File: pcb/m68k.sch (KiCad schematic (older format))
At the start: 120 parts, among them J1 USB_B_Micro, J2 Mini-DIN-6, J4 DB15_Male_HighDensity, J5 FTSH-105-01-L-DV-K, J6 FTSH-105-01-L-DV-K, J7 FTSH-105-01-L-DV-K, J8 Micro_SD_Card, U1 93LC56, U10 25LCxxx, U11 TXB0108DQSR, U12 TXB0108DQSR, U13 iCE40-HX4K-TQ144, U14 ADV7125KSTZ50, U15 74LVC1G17, U16 LD1117S33TR_SOT223, U17 LD1117S12TR_SOT223, U18 ATL431BQDBZR, U2 68000D, U3 FT2232H, U4 TXB0108DQSR, U5 TXB0108DQSR, U6 TXB0108DQSR, U7 SN74LVC8T245PWR, U8 SN74LVC8T245PWR, U9 AS6C1616, X1 ASV-12.000MHz

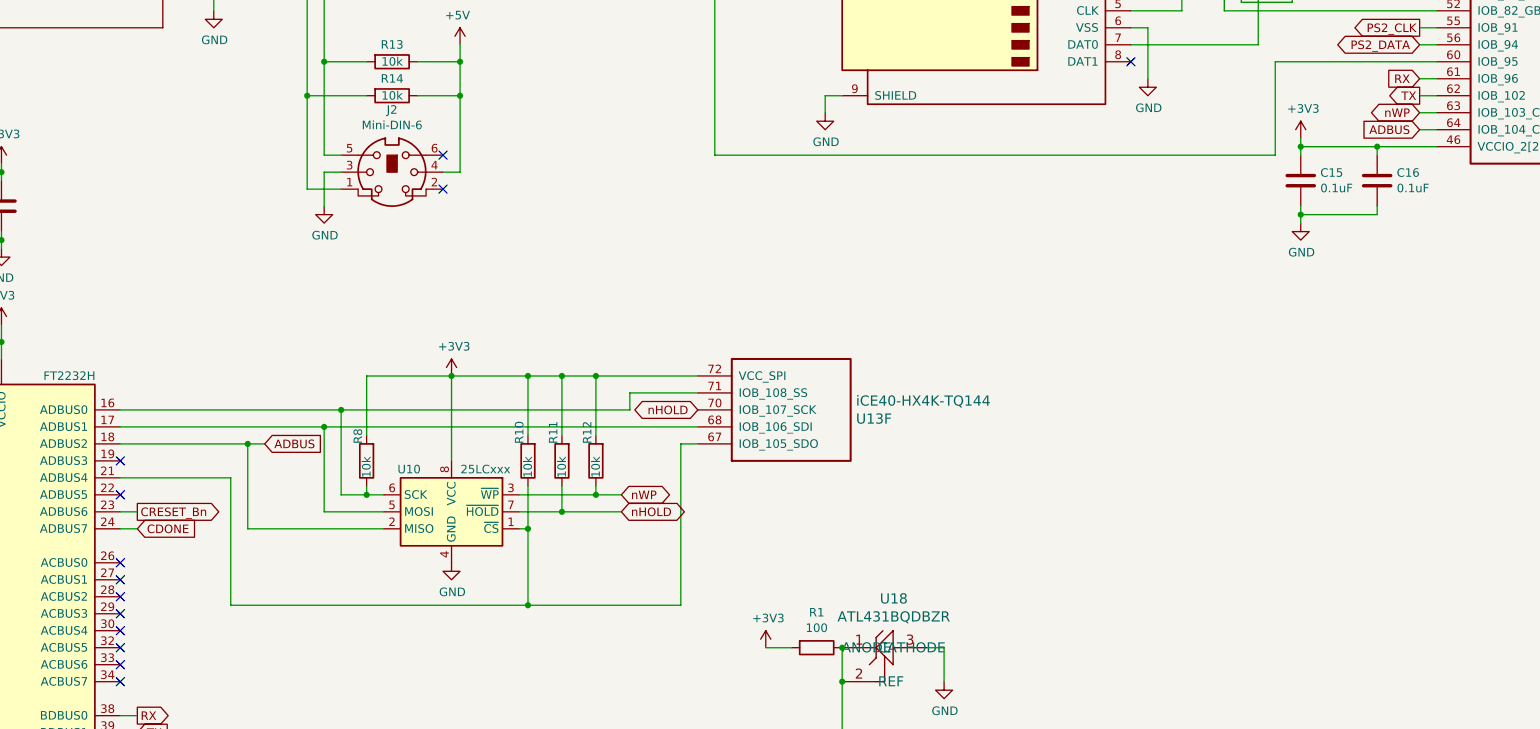
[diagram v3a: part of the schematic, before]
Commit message: almost finish routing
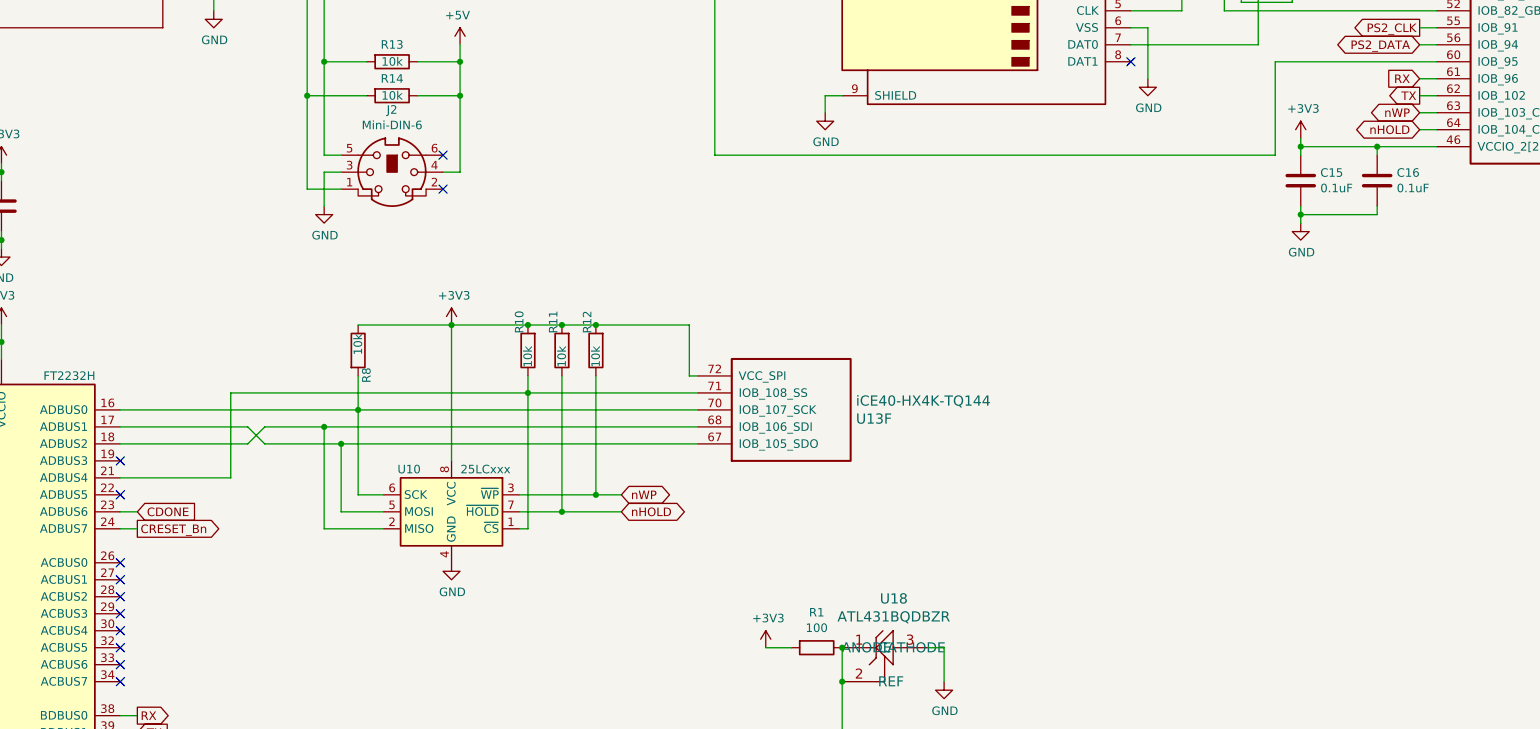
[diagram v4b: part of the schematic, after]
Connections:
- net +3V3: now also R8.1; no longer R8.2
- net CDONE: now also U3.23 (ADBUS6); no longer U3.24 (ADBUS7)
- net CRESET_Bn: now also U3.24 (ADBUS7); no longer U3.23 (ADBUS6)
- net nHOLD: now also U13.64 (IOB_104_CBSEL1); no longer U13.70 (IOB_107_SCK)
- net at R10.1, U10.1 (~CS), U3.21 (ADBUS4): now also U13.71 (IOB_108_SS); no longer U13.67 (IOB_105_SDO)
- net at U10.5 (MOSI), U3.17 (ADBUS1): now also U13.67 (IOB_105_SDO); no longer U13.68 (IOB_106_SDI)
- net at U10.6 (SCK), U3.16 (ADBUS0): now also R8.2, U13.70 (IOB_107_SCK); no longer R8.1, U13.71 (IOB_108_SS)
- net ADBUS: no longer names the net of U10.2 (MISO), U3.18 (ADBUS2)
- net ADBUS: now also U13.68 (IOB_106_SDI); no longer U13.64 (IOB_104_CBSEL1)
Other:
- moved on the sheet: R10, R11, R12, R8
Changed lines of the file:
@@
 Wire Wire Line
 	7200 3500 8050 3500
-Text GLabel 5450 12500 2    50   Input ~ 0
+Text GLabel 5450 12400 2    50   Input ~ 0
 CDONE
 Wire Wire Line
@@
 Wire Wire Line
 	8400 6300 8400 6350
-Text GLabel 13000 10150 0    50   Input ~ 0
-ADBUS
 Wire Wire Line
 	11300 9150 11850 9150
@@
 Wire Wire Line
 	8550 6400 8500 6400
-Wire Wire Line
-	6650 12300 6650 11800
-Text GLabel 6200 12000 2    50   Input ~ 0
-ADBUS
 $Comp
 L Memory_EEPROM:25LCxxx U10
@@
 	1    0    0    -1
 $EndComp
-Text GLabel 5450 12400 2    50   Output ~ 0
+Text GLabel 5450 12500 2    50   Output ~ 0
 CRESET_Bn
 Text GLabel 8300 12300 2    50   BiDi ~ 0
 nWP
-Wire Wire Line
-	7300 12100 7300 11600
-Text GLabel 8750 11800 0    50   BiDi ~ 0
+Text GLabel 13000 10150 0    50   BiDi ~ 0
 nHOLD
 $Comp
 L Device:R R12
 U 1 1 62339B13
-P 8150 12100
-F 0 "R12" V 8200 12000 50  0000 R CNN
-F 1 "10k" V 8150 12200 50  0000 R CNN
-F 2 "Resistor_SMD:R_0603_1608Metric" V 8080 12100 50  0001 C CNN
-F 3 "~" H 8150 12100 50  0001 C CNN
-	1    8150 12100
+P 8150 11450
+F 0 "R12" V 8200 11350 50  0000 R CNN
+F 1 "10k" V 8150 11550 50  0000 R CNN
+F 2 "Resistor_SMD:R_0603_1608Metric" V 8080 11450 50  0001 C CNN
+F 3 "~" H 8150 11450 50  0001 C CNN
+	1    8150 11450
 	-1   0    0    1
 $EndComp
@@
 L Device:R R11
 U 1 1 6233983C
-P 7950 12100
-F 0 "R11" V 8000 12000 50  0000 R CNN
-F 1 "10k" V 7950 12200 50  0000 R CNN
-F 2 "Resistor_SMD:R_0603_1608Metric" V 7880 12100 50  0001 C CNN
-F 3 "~" H 7950 12100 50  0001 C CNN
-	1    7950 12100
+P 7950 11450
+F 0 "R11" V 8000 11350 50  0000 R CNN
+F 1 "10k" V 7950 11550 50  0000 R CNN
+F 2 "Resistor_SMD:R_0603_1608Metric" V 7880 11450 50  0001 C CNN
+F 3 "~" H 7950 11450 50  0001 C CNN
+	1    7950 11450
 	-1   0    0    1
 $EndComp
@@
 L power:+3V3 #PWR0125
 U 1 1 605A3C62
-P 7300 11600
-F 0 "#PWR0125" H 7300 11450 50  0001 C CNN
-F 1 "+3V3" H 7315 11773 50  0000 C CNN
-F 2 "" H 7300 11600 50  0001 C CNN
-F 3 "" H 7300 11600 50  0001 C CNN
-	1    7300 11600
+P 7300 11300
+F 0 "#PWR0125" H 7300 11150 50  0001 C CNN
+F 1 "+3V3" H 7315 11473 50  0000 C CNN
+F 2 "" H 7300 11300 50  0001 C CNN
+F 3 "" H 7300 11300 50  0001 C CNN
+	1    7300 11300
 	1    0    0    -1
 $EndComp
@@
 L Device:R R8
 U 1 1 605A381A
-P 6800 12100
-F 0 "R8" V 6850 12000 50  0000 R CNN
-F 1 "10k" V 6800 12200 50  0000 R CNN
-F 2 "Resistor_SMD:R_0603_1608Metric" V 6730 12100 50  0001 C CNN
-F 3 "~" H 6800 12100 50  0001 C CNN
-	1    6800 12100
-	-1   0    0    1
+P 6750 11450
+F 0 "R8" V 6800 11350 50  0000 R CNN
+F 1 "10k" V 6750 11550 50  0000 R CNN
+F 2 "Resistor_SMD:R_0603_1608Metric" V 6680 11450 50  0001 C CNN
+F 3 "~" H 6750 11450 50  0001 C CNN
+	1    6750 11450
+	1    0    0    -1
 $EndComp
 $Comp
 L Device:R R10
 U 1 1 605A28F2
-P 7750 12100
-F 0 "R10" V 7800 12000 50  0000 R CNN
-F 1 "10k" V 7750 12200 50  0000 R CNN
-F 2 "Resistor_SMD:R_0603_1608Metric" V 7680 12100 50  0001 C CNN
-F 3 "~" H 7750 12100 50  0001 C CNN
-	1    7750 12100
+P 7750 11450
+F 0 "R10" V 7800 11350 50  0000 R CNN
+F 1 "10k" V 7750 11550 50  0000 R CNN
+F 2 "Resistor_SMD:R_0603_1608Metric" V 7680 11450 50  0001 C CNN
+F 3 "~" H 7750 11450 50  0001 C CNN
+	1    7750 11450
 	-1   0    0    1
 $EndComp
 Wire Wire Line
-	6550 11900 6550 12400
-Wire Wire Line
 	7700 12300 8150 12300
 Wire Wire Line
 	7700 12400 7950 12400
 Wire Wire Line
-	8150 11950 8150 11600
-Wire Wire Line
-	7950 11950 7950 11600
-Wire Wire Line
-	7950 11600 8150 11600
-Connection ~ 8150 11600
-Wire Wire Line
-	7750 11950 7750 11600
-Wire Wire Line
-	7750 11600 7950 11600
-Connection ~ 7950 11600
-Wire Wire Line
-	7750 12250 7750 12500
-Wire Wire Line
-	7950 12250 7950 12400
-Wire Wire Line
-	6100 12000 6100 12500
-Connection ~ 6100 12000
-Wire Wire Line
-	6100 12000 6200 12000
-Wire Wire Line
 	5350 12200 6000 12200
-Wire Wire Line
-	5350 12000 6100 12000
-Wire Wire Line
-	6000 12200 6000 12950
-Wire Wire Line
-	7750 12500 7750 12950
-Connection ~ 7750 12500
 Connection ~ 7950 12400
 Text GLabel 8300 12400 2    50   BiDi ~ 0
@@
 Wire Wire Line
 	7950 12400 8300 12400
-Wire Wire Line
-	8150 12250 8150 12300
 Connection ~ 8150 12300
 Wire Wire Line
 	8150 12300 8300 12300
 Wire Wire Line
-	8650 12000 8650 12950
-Connection ~ 7750 11600
-Connection ~ 7300 11600
-Connection ~ 7750 12950
-Wire Wire Line
-	6000 12950 7750 12950
-Connection ~ 6550 11900
-Wire Wire Line
-	6800 11950 6800 11600
-Wire Wire Line
-	6800 11600 7300 11600
-Wire Wire Line
-	8350 11800 8350 11700
-Connection ~ 6650 11800
-Wire Wire Line
-	6800 12250 6800 12300
-Wire Wire Line
-	6800 12300 6900 12300
-Wire Wire Line
-	6650 12300 6800 12300
-Connection ~ 6800 12300
-Wire Wire Line
-	6550 12400 6900 12400
-Wire Wire Line
-	6100 12500 6900 12500
-Wire Wire Line
-	7750 12950 8650 12950
-Wire Wire Line
-	8650 12000 8750 12000
-Wire Wire Line
-	8150 11600 8750 11600
-Wire Wire Line
-	6550 11900 8750 11900
-Wire Wire Line
-	5350 11800 6650 11800
-Wire Wire Line
-	7300 11600 7750 11600
-Wire Wire Line
-	5350 11900 6550 11900
-Wire Wire Line
-	8350 11700 8750 11700
-Wire Wire Line
-	6650 11800 8350 11800
-Wire Wire Line
 	12150 10300 12150 9750
 Wire Wire Line
@@
 Wire Wire Line
 	7750 8750 8150 8750
+Wire Wire Line
+	5350 11800 6750 11800
+Wire Wire Line
+	6000 12200 6000 11700
+Wire Wire Line
+	6000 11700 7750 11700
+Wire Wire Line
+	5350 12000 6100 12000
+Wire Wire Line
+	5350 11900 6100 11900
+Wire Wire Line
+	6100 11900 6200 12000
+Wire Wire Line
+	6100 12000 6200 11900
+Wire Wire Line
+	6200 11900 6550 11900
+Wire Wire Line
+	6200 12000 6650 12000
+Wire Wire Line
+	6900 12300 6750 12300
+Wire Wire Line
+	6750 12300 6750 11800
+Connection ~ 6750 11800
+Wire Wire Line
+	6750 11800 8750 11800
+Wire Wire Line
+	6900 12400 6650 12400
+Wire Wire Line
+	6650 12400 6650 12000
+Connection ~ 6650 12000
+Wire Wire Line
+	6650 12000 8750 12000
+Wire Wire Line
+	6900 12500 6550 12500
+Wire Wire Line
+	6550 12500 6550 11900
+Connection ~ 6550 11900
+Wire Wire Line
+	6550 11900 8750 11900
+Wire Wire Line
+	7750 11700 7750 12500
+Connection ~ 7750 11700
+Wire Wire Line
+	7750 11700 8750 11700
+Connection ~ 7750 11300
+Connection ~ 7950 11300
+Connection ~ 8150 11300
+Wire Wire Line
+	8150 11300 8700 11300
+Wire Wire Line
+	7750 11300 7950 11300
+Wire Wire Line
+	7950 11300 8150 11300
+Wire Wire Line
+	7950 11600 7950 12400
+Wire Wire Line
+	7750 11700 7750 11600
+Wire Wire Line
+	8150 11600 8150 12300
+Wire Wire Line
+	6750 11800 6750 11600
+Wire Wire Line
+	8700 11300 8700 11600
+Wire Wire Line
+	8700 11600 8750 11600
+Wire Wire Line
+	7300 12100 7300 11300
+Connection ~ 7300 11300
+Wire Wire Line
+	7300 11300 7750 11300
+Wire Wire Line
+	6750 11300 7300 11300
 Wire Bus Line
 	18600 2100 18600 2800

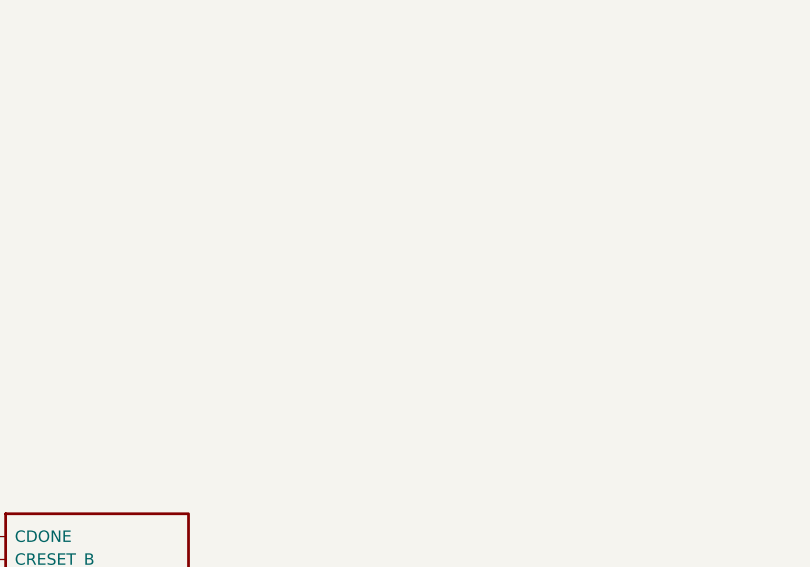
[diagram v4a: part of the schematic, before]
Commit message: vanity
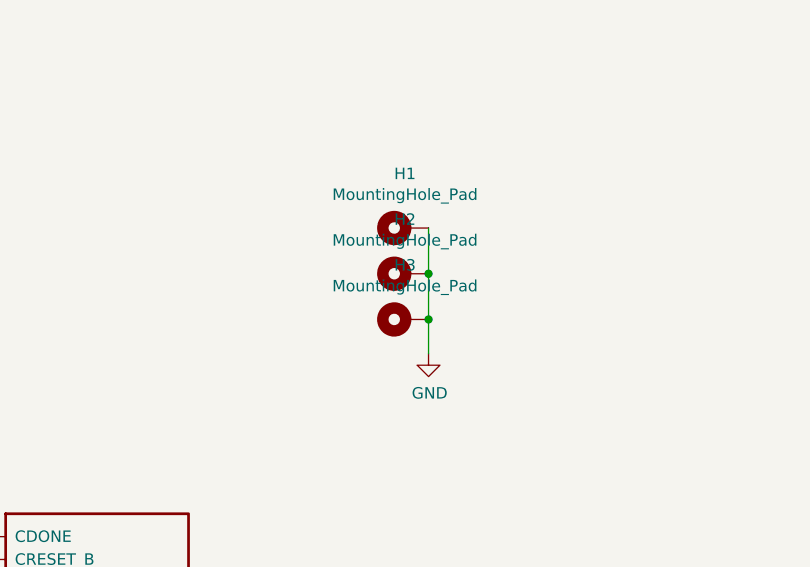
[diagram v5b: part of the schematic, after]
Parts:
- added H1, H2, H3: MountingHole_Pad, MountingHole:MountingHole_2.5mm_Pad, symbol Mechanical:MountingHole_Pad
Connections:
- net GND: now also H1.1, H2.1, H3.1
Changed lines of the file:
@@
 Wire Wire Line
 	6750 11300 7300 11300
+Wire Wire Line
+	15150 6800 15150 7000
+Connection ~ 15150 7000
+Wire Wire Line
+	15150 7000 15150 7200
+Connection ~ 15150 7200
+Wire Wire Line
+	15150 7200 15150 7350
+$Comp
+L power:GND #PWR06
+U 1 1 5EA04520
+P 15150 7350
+F 0 "#PWR06" H 15150 7100 50  0001 C CNN
+F 1 "GND" H 15155 7177 50  0000 C CNN
+F 2 "" H 15150 7350 50  0001 C CNN
+F 3 "" H 15150 7350 50  0001 C CNN
+	1    15150 7350
+	1    0    0    -1
+$EndComp
+$Comp
+L Mechanical:MountingHole_Pad H1
+U 1 1 5EA6048F
+P 15050 6800
+F 0 "H1" V 15287 6803 50  0000 C CNN
+F 1 "MountingHole_Pad" V 15196 6803 50  0000 C CNN
+F 2 "MountingHole:MountingHole_2.5mm_Pad" H 15050 6800 50  0001 C CNN
+F 3 "~" H 15050 6800 50  0001 C CNN
+	1    15050 6800
+	0    -1   -1   0
+$EndComp
+$Comp
+L Mechanical:MountingHole_Pad H2
+U 1 1 5EA61D1E
+P 15050 7000
+F 0 "H2" V 15287 7003 50  0000 C CNN
+F 1 "MountingHole_Pad" V 15196 7003 50  0000 C CNN
+F 2 "MountingHole:MountingHole_2.5mm_Pad" H 15050 7000 50  0001 C CNN
+F 3 "~" H 15050 7000 50  0001 C CNN
+	1    15050 7000
+	0    -1   -1   0
+$EndComp
+$Comp
+L Mechanical:MountingHole_Pad H3
+U 1 1 5EA63D7B
+P 15050 7200
+F 0 "H3" V 15287 7203 50  0000 C CNN
+F 1 "MountingHole_Pad" V 15196 7203 50  0000 C CNN
+F 2 "MountingHole:MountingHole_2.5mm_Pad" H 15050 7200 50  0001 C CNN
+F 3 "~" H 15050 7200 50  0001 C CNN
+	1    15050 7200
+	0    -1   -1   0
+$EndComp
 Wire Bus Line
 	18600 2100 18600 2800
